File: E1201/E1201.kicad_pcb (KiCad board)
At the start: 2 copper layers, 83.8 x 43.1 mm, 53 parts, among them J1 Screw_Terminal_01x02, J2 Screw_Terminal_01x04, J3 Conn_01x04_Socket, J4 Conn_01x06_Socket, J6 Conn_02x08_Odd_Even, J7 Conn_01x18, J8 ICSP, J9 QWIIC, Q1 MMBF170, Q2 MMBF170, Q3 MMBF170, SW1 SW_Push, U1 TXU0304PW, U2 TXU0202DCU, U3 TCA9517ADGK, U4 TPS61222DCK, U5 PIC16F18154-xSTX, U6 LM2776

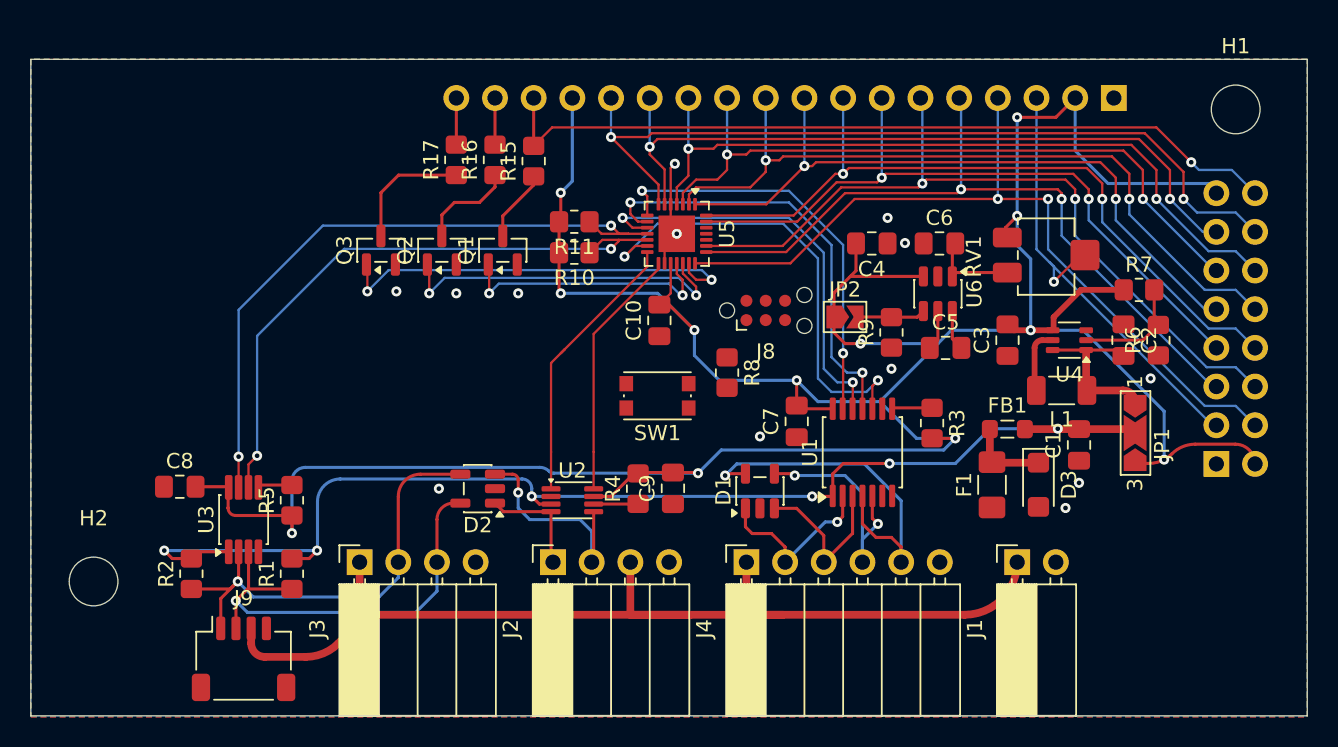
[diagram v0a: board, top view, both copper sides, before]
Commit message: PCB Commit, this is what I used to order
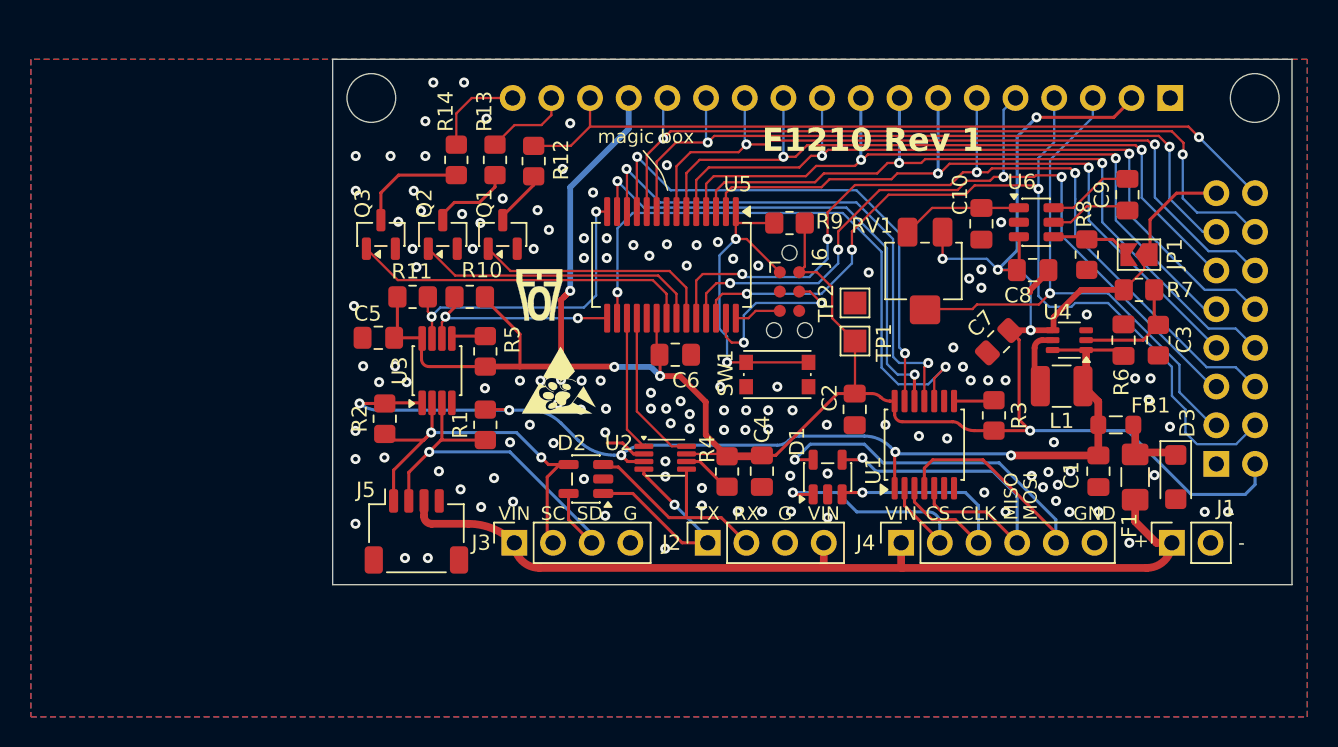
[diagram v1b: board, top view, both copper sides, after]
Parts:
- removed the JP1 at (201.4, 87.0)
- added TP1: TestPoint, TestPoint:TestPoint_Pad_1.5x1.5mm, F.Cu at (183.0, 81.0)
- added TP2: TestPoint, TestPoint:TestPoint_Pad_1.5x1.5mm, F.Cu at (183.0, 78.5)
- C3: renamed from C2; value C -> 10uF
- C7: renamed from C3; value C -> 10uF
- J1: footprint Connector_PinSocket_2.54mm:PinSocket_1x02_P2.54mm_Horizontal -> Connector_PinSocket_2.54mm:PinSocket_1x02_P2.54mm_Vertical
- J2: value Screw_Terminal_01x04 -> Conn_01x04_Socket; footprint Connector_PinSocket_2.54mm:PinSocket_1x04_P2.54mm_Horizontal -> Connector_PinSocket_2.54mm:PinSocket_1x04_P2.54mm_Vertical
- J3: footprint Connector_PinSocket_2.54mm:PinSocket_1x04_P2.54mm_Horizontal -> Connector_PinSocket_2.54mm:PinSocket_1x04_P2.54mm_Vertical
- J4: footprint Connector_PinSocket_2.54mm:PinSocket_1x06_P2.54mm_Horizontal -> Connector_PinSocket_2.54mm:PinSocket_1x06_P2.54mm_Vertical
- L1: value L -> 4.7uH; footprint Inductor_SMD:L_1206_3216Metric_Pad1.22x1.90mm_HandSolder -> Inductor_SMD:L_1210_3225Metric
- R6: value 10k -> 20k
- R7: value 10k -> 180k
- U5: value PIC16F18154-xSTX -> PIC16F18154-xSP; footprint Package_DFN_QFN:QFN-28-1EP_4x4mm_P0.4mm_EP2.4x2.4mm -> Package_SO:SSOP-28_5.3x10.2mm_P0.65mm
- moved H2 36.6 mm to (151.2, 65.0)
- moved JP1 19.7 mm to (201.7, 75.3), turned to 180 degrees
- moved C5 16.3 mm to (151.7, 80.7)
- moved R2 16.3 mm to (152.1, 86.1)
- moved U3 16.0 mm to (155.6, 82.9)
- moved R1 16.0 mm to (158.7, 86.5)
- moved R5 16.0 mm to (158.7, 81.6)
- moved C9 15.6 mm to (200.9, 71.3), turned to 90 degrees
- moved J5 14.1 mm to (154.2, 93.5)
- moved R8 13.8 mm to (198.2, 75.3)
- moved R11 11.7 mm to (153.9, 78.1)
- moved C8 10.7 mm to (194.7, 76.3)
- moved R9 10.6 mm to (178.7, 73.2), turned to 0 degrees
- moved J2 10.2 mm to (173.3, 94.2)
- moved J1 10.2 mm to (203.8, 94.2)
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- renumbered C6 to C10, C7 to C2, C9 to C4, C8 to C5, C10 to C6, C4 to C8, C5 to C9, J9 to J5, J8 to J6, J6 to J7, J7 to J8, JP2 to JP1, R15 to R12, R16 to R13, R17 to R14, R9 to R8, R8 to R9
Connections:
- C3 pad 2: Net-(JP1-A) -> VIN-P
- J2 pad 3: VIN -> GND
- J2 pad 4: GND -> VIN
- J6 pad 1: /PROG_RST -> /PROG_VPP
- L1 pad 1: Net-(JP1-A) -> VIN-P
- R9 pad 1: /PROG_RST -> /PROG_VPP
- SW1 pad 2: /PROG_RST -> /PROG_VPP
- U4 pad 1: Net-(JP1-A) -> VIN-P
- U4 pad 6: Net-(JP1-A) -> VIN-P
- U5 pad 1: /LCD_{D2} -> /PROG_VPP
- U5 pad 10: /MCU_SPI_CLK -> /LCD_{D7}
- U5 pad 11: /MCU_I2C_SCL -> /MCU_SPI_~{CS}
- U5 pad 12: /MCU_I2C_SDA -> /MCU_SPI_MOSI
- U5 pad 13: /MCU_SPI_MISO -> /MCU_SPI_CLK
- U5 pad 14: /MCU_UART_TX -> /MCU_I2C_SCL
- U5 pad 15: /MCU_UART_RX -> /MCU_I2C_SDA
- U5 pad 16: GND -> /MCU_SPI_MISO
- U5 pad 17: +5V -> /MCU_UART_TX
- U5 pad 18: /LCD_{BL_{1}}_EN -> /MCU_UART_RX
- U5 pad 19: /LCD_{BL_{2}}_EN -> GND
- U5 pad 2: /LCD_{D3} -> /LCD_{D0}
- U5 pad 20: /LCD_{BL_{3}}_EN -> +5V
- U5 pad 21: /LCD_{RS} -> /LCD_{BL_{3}}_EN
- U5 pad 22: /LCD_{RW} -> /LCD_{BL_{2}}_EN
- U5 pad 23: /LCD_{EN} -> /LCD_{BL_{1}}_EN
- U5 pad 24: /PROG_CLK -> /LCD_{EN}
- U5 pad 25: /PROG_DAT -> /LCD_{RW}
- U5 pad 26: /PROG_RST -> /LCD_{RS}
- U5 pad 27: /LCD_{D0} -> /PROG_CLK
- U5 pad 28: /LCD_{D1} -> /PROG_DAT
- U5 pad 3: /LCD_{D4} -> /LCD_{D1}
- U5 pad 4: /LCD_{D5} -> /LCD_{D2}
- U5 pad 5: GND -> /LCD_{D3}
- U5 pad 6: /LCD_{D6} -> /LCD_{D4}
- U5 pad 7: /LCD_{D7} -> /LCD_{D5}
- U5 pad 8: /MCU_SPI_~{CS} -> GND
- U5 pad 9: /MCU_SPI_MOSI -> /LCD_{D6}
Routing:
- net +5V: track 217.6 -> 175.6 mm, vias 12 -> 8
- net /MCU_I2C_SDA: track 40.7 -> 13.8 mm
- net /MCU_I2C_SCL: track 43.9 -> 20.3 mm
- net /PROG_VPP: track 0.00 -> 22.2 mm, vias 0 -> 2
- net VIN: track 71.8 -> 60.2 mm
- net /PROG_CLK: track 0.00 -> 11.6 mm, vias 0 -> 2
- net Net-(JP1-A): track 11.0 -> 0.00 mm
- net /SPI_MOSI: track 24.3 -> 35.2 mm
- net VIN-P: track 81.8 -> 71.5 mm, vias 6 -> 5
- net /MCU_UART_TX: track 18.5 -> 8.87 mm
- net /MCU_SPI_MISO: track 30.8 -> 40.0 mm
- net /LCD_{RS}: track 53.2 -> 61.1 mm, vias 2 -> 3
- net /SPI_MISO: track 15.8 -> 23.0 mm, vias 2 -> 1
- net /LCD_{BIAS}: track 30.7 -> 37.9 mm
- net /UART_TX: track 7.28 -> 14.5 mm, vias 0 -> 1
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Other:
- board size 83.8 x 43.1 mm -> 63 x 34.5 mm
- board text added: "+"
- board text added: "-"
- board text added: "CLK"
- board text added: "CS"
- board text added: "E1210 Rev 1"
- board text added: "E1210 Rev 1 Generic LCD Backback"
- board text added: "G"
- board text added: "GND"
- board text added: "MISO"
- board text added: "MOSI"
- board text added: "RX"
- board text added: "SC"
- board text added: "SD"
- board text added: "TX"
- board text added: "VIN"
- board text added: "magic box"
